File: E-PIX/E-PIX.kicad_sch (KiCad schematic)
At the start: 45 parts, among them J1 USB_C_Receptacle_USB2.0, J2 BNO055, J3 ADC, J4 ADC, Q1 BSS138, Q2 BSS138, SW1 SW, SW2 SW_Push, U1 Conn_03x04, U2 Conn_03x04, U3 TC7WH241FK, U4 TC7WH241FK, U5 NJM7805SDL1, U6 AZ1117-3.3, U7 ESP32-C3-WROOM-02, U8 BTS6142D

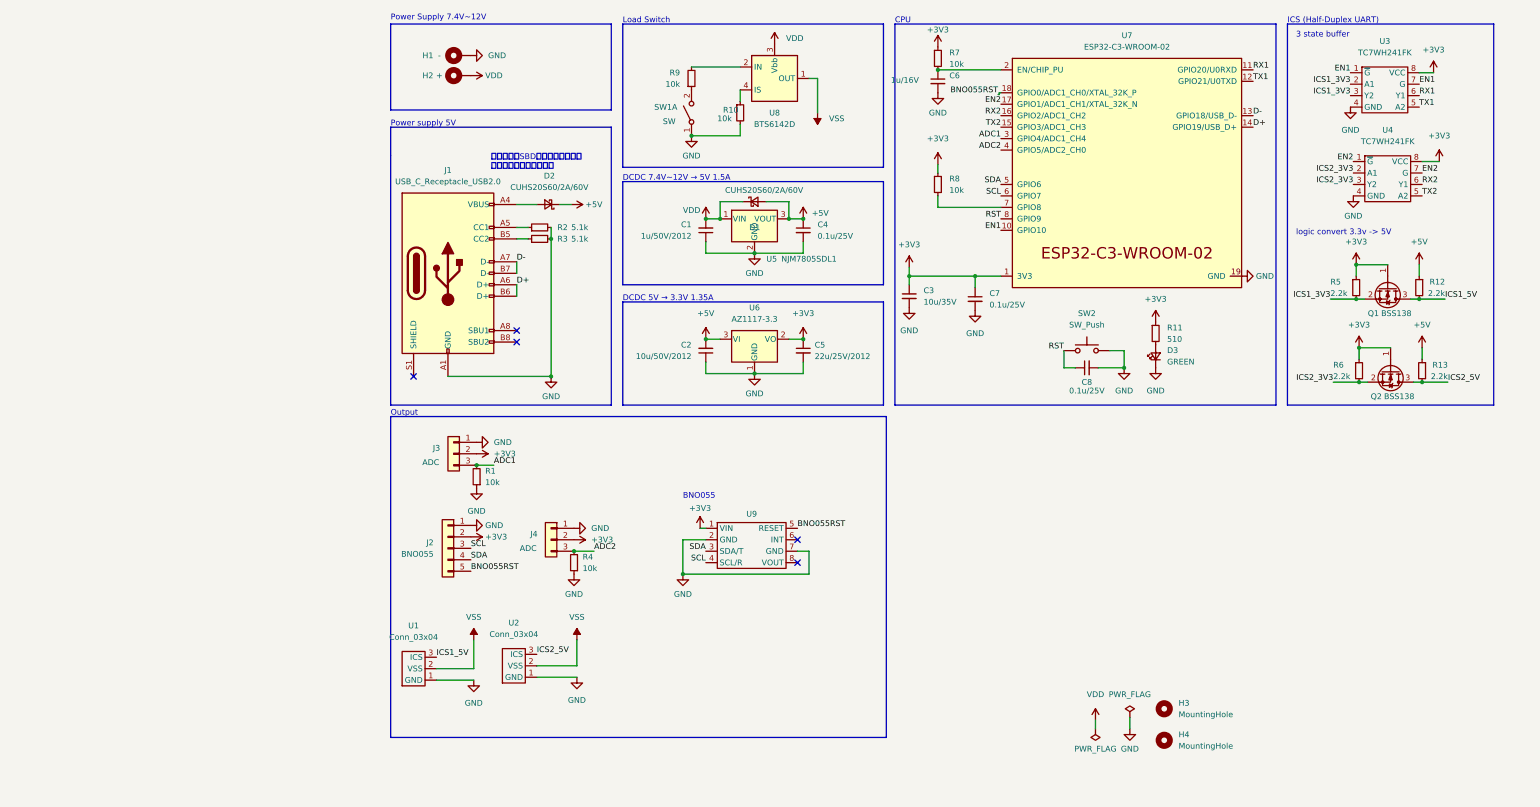
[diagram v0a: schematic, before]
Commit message: add SD card mod
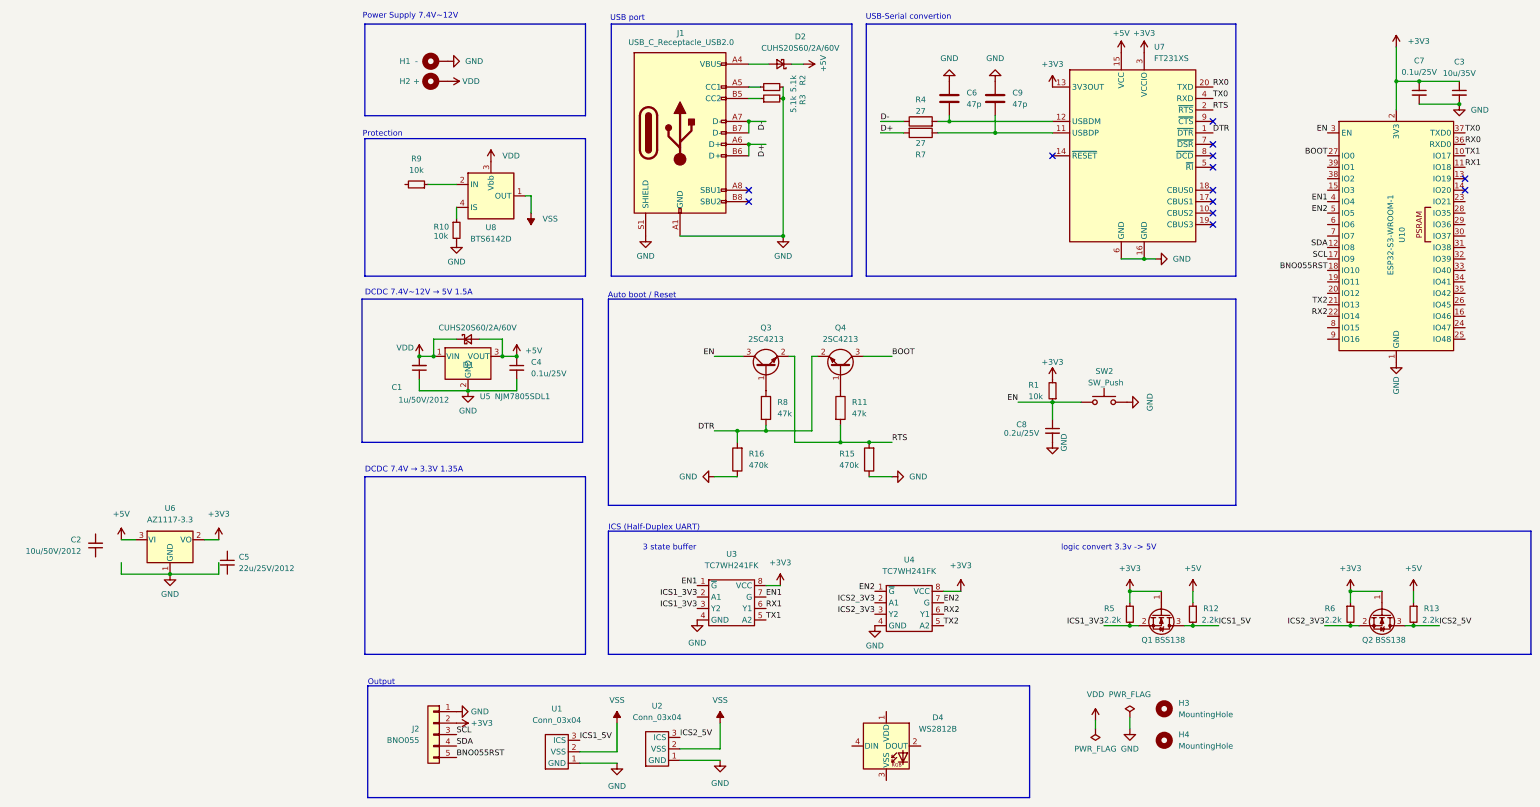
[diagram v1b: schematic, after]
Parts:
- removed C6: 1u/16V, Capacitor_SMD:C_0603_1608Metric, symbol Device:C_Small
- removed D3: GREEN, LED_SMD:LED_0603_1608Metric, symbol Device:LED_Small
- removed J3, J4: ADC, Connector_PinHeader_2.54mm:PinHeader_1x03_P2.54mm_Vertical, symbol Connector_Generic:Conn_01x03
- removed R11: 510, Resistor_SMD:R_0603_1608Metric, symbol Device:R_Small
- removed R4, R7, R8: 10k, Resistor_SMD:R_0603_1608Metric, symbol Device:R_Small
- removed SW1: SW, Connector_PinHeader_2.54mm:PinHeader_1x02_P2.54mm_Vertical, symbol Switch:SW_DPST_x2
- removed U7: ESP32-C3-WROOM-02, Espressif:ESP32-C3-WROOM-02, symbol Espressif:ESP32-C3-WROOM-02
- removed U9: ~, IMU:BNO055, symbol IMU:BNO055
- added C6, C9: 47p, symbol Device:C
- added D4: WS2812B, LED_SMD:LED_WS2812B_PLCC4_5.0x5.0mm_P3.2mm, symbol LED:WS2812B
- added Q3, Q4: 2SC4213, Package_TO_SOT_SMD:SOT-323_SC-70, symbol Transistor_BJT:2SC4213
- added R11, R8: 47k, symbol Device:R
- added R15, R16: 470k, symbol Device:R
- added R4, R7: 27, symbol Device:R
- added U10: ESP32-S3-WROOM-1, RF_Module:ESP32-S3-WROOM-1, symbol RF_Module:ESP32-S3-WROOM-1
- added U7: FT231XS, Package_SO:SSOP-20_3.9x8.7mm_P0.635mm, symbol Interface_USB:FT231XS
- C8: value 0.1u/25V -> 0.2u/25V
- J2: footprint Connector_PinHeader_2.54mm:PinHeader_1x05_P2.54mm_Vertical -> Connector_JST:JST_XH_B4B-XH-A_1x04_P2.50mm_Vertical
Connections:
- net ADC1 is gone; now on net +3V3: R1.2
- net +3V3: now also U10.2 (3V3), U7.13 (3V3OUT), U7.3 (VCCIO); no longer C5.1
- net +5V: now also U7.15 (VCC); no longer C2.2
- net BNO055RST: now also U10.18 (IO10)
- net D+: now also R7.2
- net D-: now also R4.1
- net EN1: now also U10.4 (IO4)
- net EN2: now also U10.5 (IO5)
- net GND: now also J1.S1 (SHIELD), C6.1, C9.1, R15.1, R16.1, U10.1 (GND), U10.40 (GND), U10.41 (GND), U7.16 (GND), U7.6 (GND); no longer C2.1, C5.2, R1.1
- net RX1: now also U10.11 (IO18)
- net RX2: now also U10.22 (IO14)
- net SCL: now also U10.17 (IO9)
- net SDA: now also U10.12 (IO8)
- net TX1: now also U10.10 (IO17)
- net TX2: now also U10.21 (IO13)
- net at R9.1: now also U8.2 (IN)
- net at R9.2: no longer U8.2 (IN)
- net RST renamed EN
- net EN: now also R1.1, Q3.3 (C), U10.3 (EN)
- new net: C9.2, R7.1, U7.11 (USBDP)
- new net: Q3.1 (B), R8.1
- new net: C6.2, R4.2, U7.12 (USBDM)
- new net: Q4.1 (B), R11.1
- new net BOOT: Q4.3 (C), U10.27 (IO0)
- new net DTR: Q4.2 (E), R16.2, R8.2, U7.1 (~{DTR})
- new net RTS: Q3.2 (E), R11.2, R15.2, U7.2 (~{RTS})
- new net RX0: U10.36 (RXD0), U7.20 (TXD)
- new net TX0: U10.37 (TXD0), U7.4 (RXD)
- no-connect marks 5 -> 13
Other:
- note added: "Auto boot / Reset"
- note added: "DCDC 7.4V → 3.3V 1.35A"
- note added: "Protection"
- note added: "USB port"
- note added: "USB-Serial convertion"
- note removed: "BNO055"
- note removed: "CPU"
- note removed: "DCDC 5V → 3.3V 1.35A"
- note removed: "Load Switch"
- note removed: "Power supply 5V"
- note removed: "逆流防止用SBD 電圧降下のため デバックにしか使わない"
- moved on the sheet: C1, C2, C3, C4, C5, C7, C8, D1, D2, H1, H2, J1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
